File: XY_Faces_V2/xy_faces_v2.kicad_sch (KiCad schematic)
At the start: 26 parts, among them CN1 DF13A-5P-1.25H(21), CN2 DF13C-5P-1.25V(21), J2 Conn_01x01, J3 Conn_01x01, J4 Conn_01x01, J5 Conn_01x01, U1 VEML7700, U2 MCP9808_DFN, U3 DRV2605LDGS

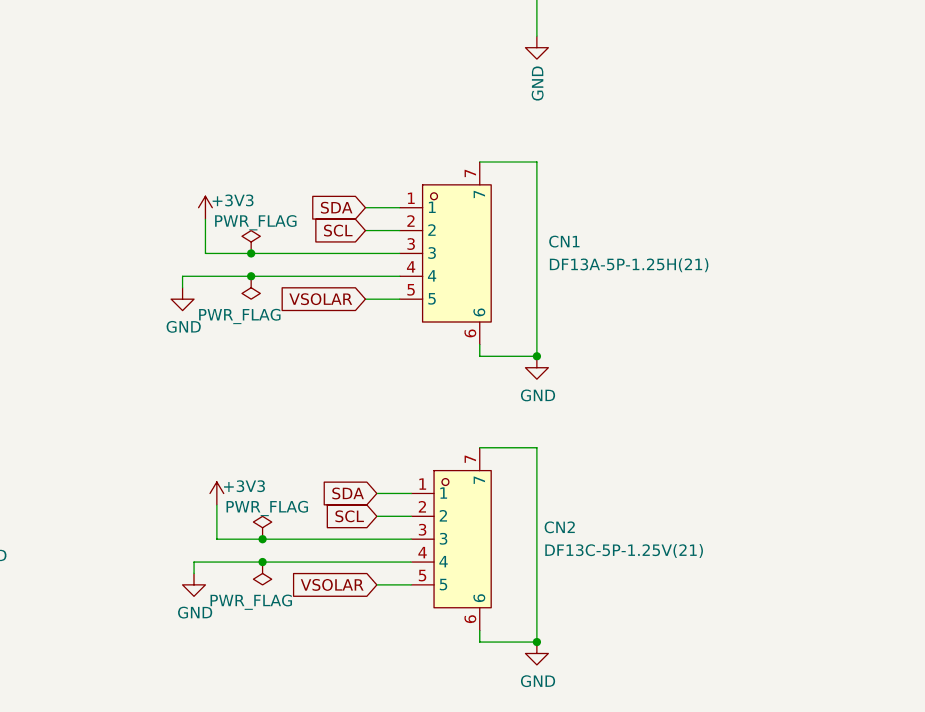
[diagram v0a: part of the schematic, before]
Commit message: updated schematic
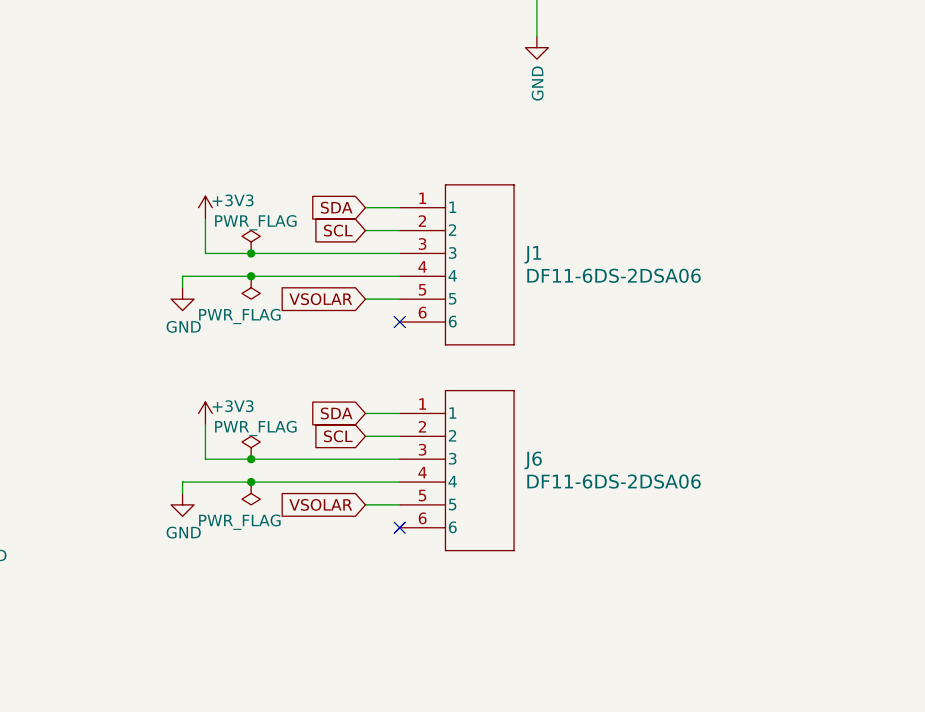
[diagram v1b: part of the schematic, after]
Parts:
- removed CN1: DF13A-5P-1.25H(21), easyeda2kicad:CONN-SMD_5P-P1.25_HRS_DF13A-5P-1.25H, symbol easyeda2kicad:DF13A-5P-1.25H(21)
- removed CN2: DF13C-5P-1.25V(21), easyeda2kicad:CONN-SMD_DF13C-5P-1.25V-21, symbol easyeda2kicad:DF13C-5P-1.25V(21)
- added J1, J6: DF11-6DS-2DSA06, CON6_2X3_U_DF11_HIR, symbol DF11-6DS-2DSA(05):DF11-6DS-2DSA06
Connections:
- net +3V3: now also J1.3, J6.3
- net GND: now also J1.4, J6.4
- net SCL: now also J1.2, J6.2
- net SDA: now also J1.1, J6.1
- net VSOLAR: now also J1.5, J6.5
- no-connect marks 6 -> 8
